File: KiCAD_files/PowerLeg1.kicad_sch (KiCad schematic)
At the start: 63 parts, among them Q301 IPD200N15N3, Q302 IPD200N15N3, Q303 IPD200N15N3, U301 AMC1100DUB, U302 ACS730xLCTR-20AB, U303 UCC21222DR, U304 OPA316, U305 OPA316, U306 SFH617A-2X009T

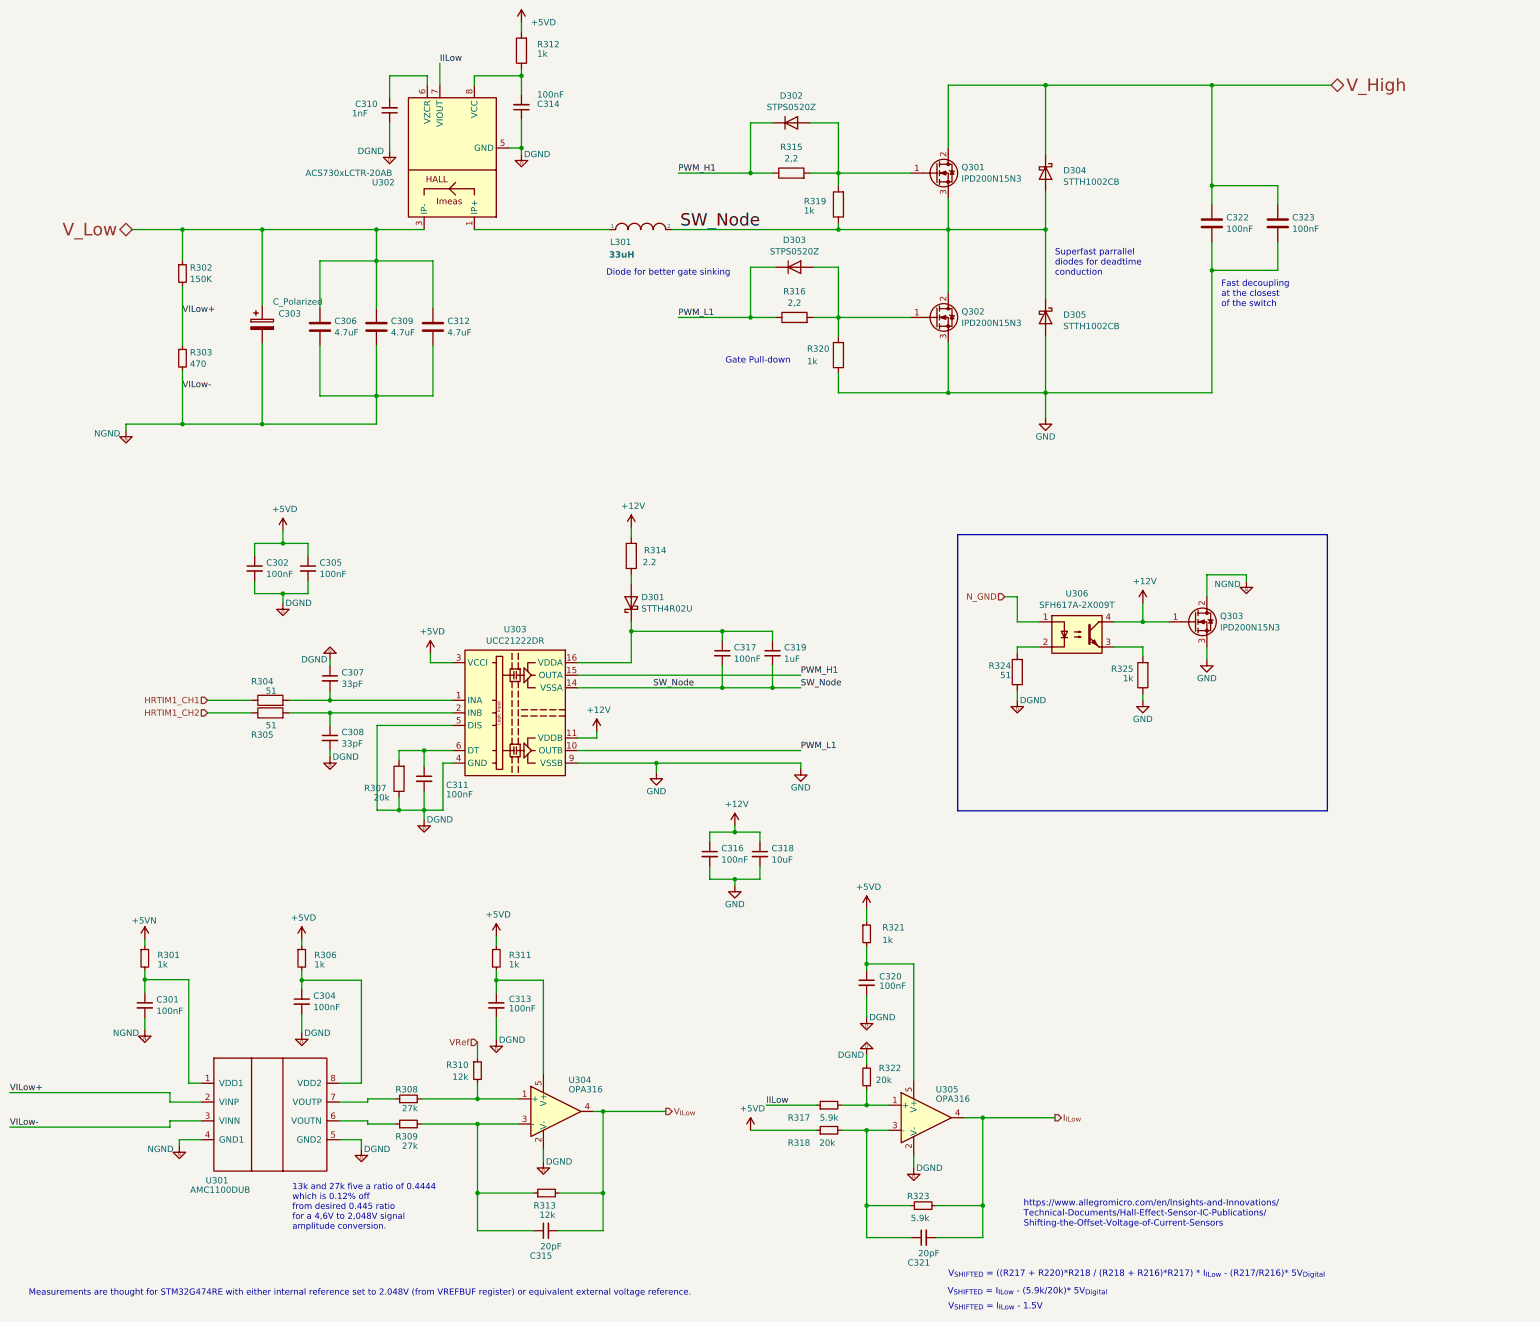
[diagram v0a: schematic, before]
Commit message: WIP: integrated the feeder on the power board directly
Former-commit-id: e81265b44c994f7ae6e14a178f616f328de7a2ab
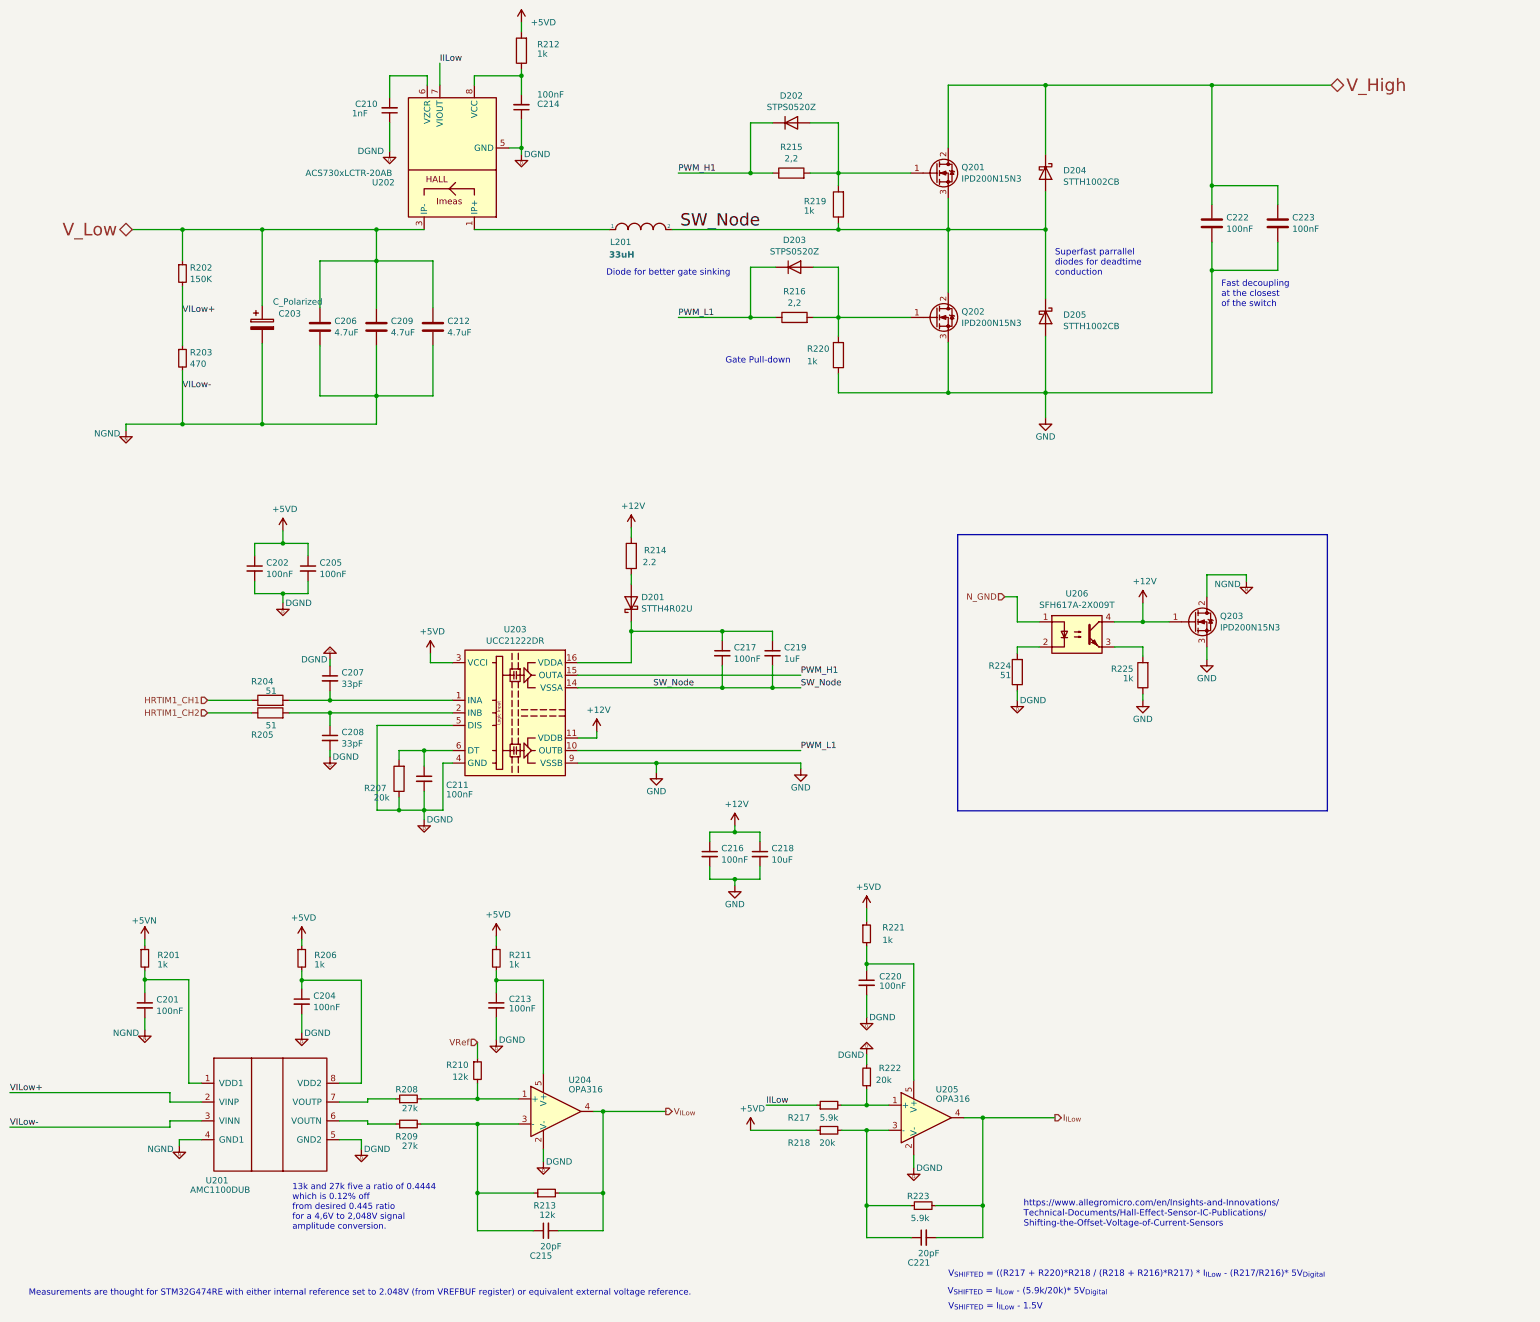
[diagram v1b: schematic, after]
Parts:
- renumbered C301 to C201, C302 to C202, C303 to C203, C304 to C204, C305 to C205, C306 to C206, C307 to C207, C308 to C208, C309 to C209, C310 to C210, C311 to C211, C312 to C212, C313 to C213, C314 to C214, C315 to C215, C316 to C216, C317 to C217, C318 to C218, C319 to C219, C320 to C220, C321 to C221, C322 to C222, C323 to C223, D301 to D201, D302 to D202, D303 to D203, D304 to D204, D305 to D205, L301 to L201, Q301 to Q201, Q302 to Q202, Q303 to Q203, R301 to R201, R302 to R202, R303 to R203, R304 to R204, R305 to R205, R306 to R206, R307 to R207, R308 to R208, R309 to R209, R310 to R210, R311 to R211, R312 to R212, R313 to R213, R314 to R214, R315 to R215, R316 to R216, R317 to R217, R318 to R218, R319 to R219, R320 to R220, R321 to R221, R322 to R222, R323 to R223, R324 to R224, R325 to R225, U301 to U201, U302 to U202, U303 to U203, U304 to U204, U305 to U205, U306 to U206

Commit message: WIP : 99 percents of the nets are now routed properly
Former-commit-id: fcbb95e3f0a6512a63faba729c3990d7109d7768
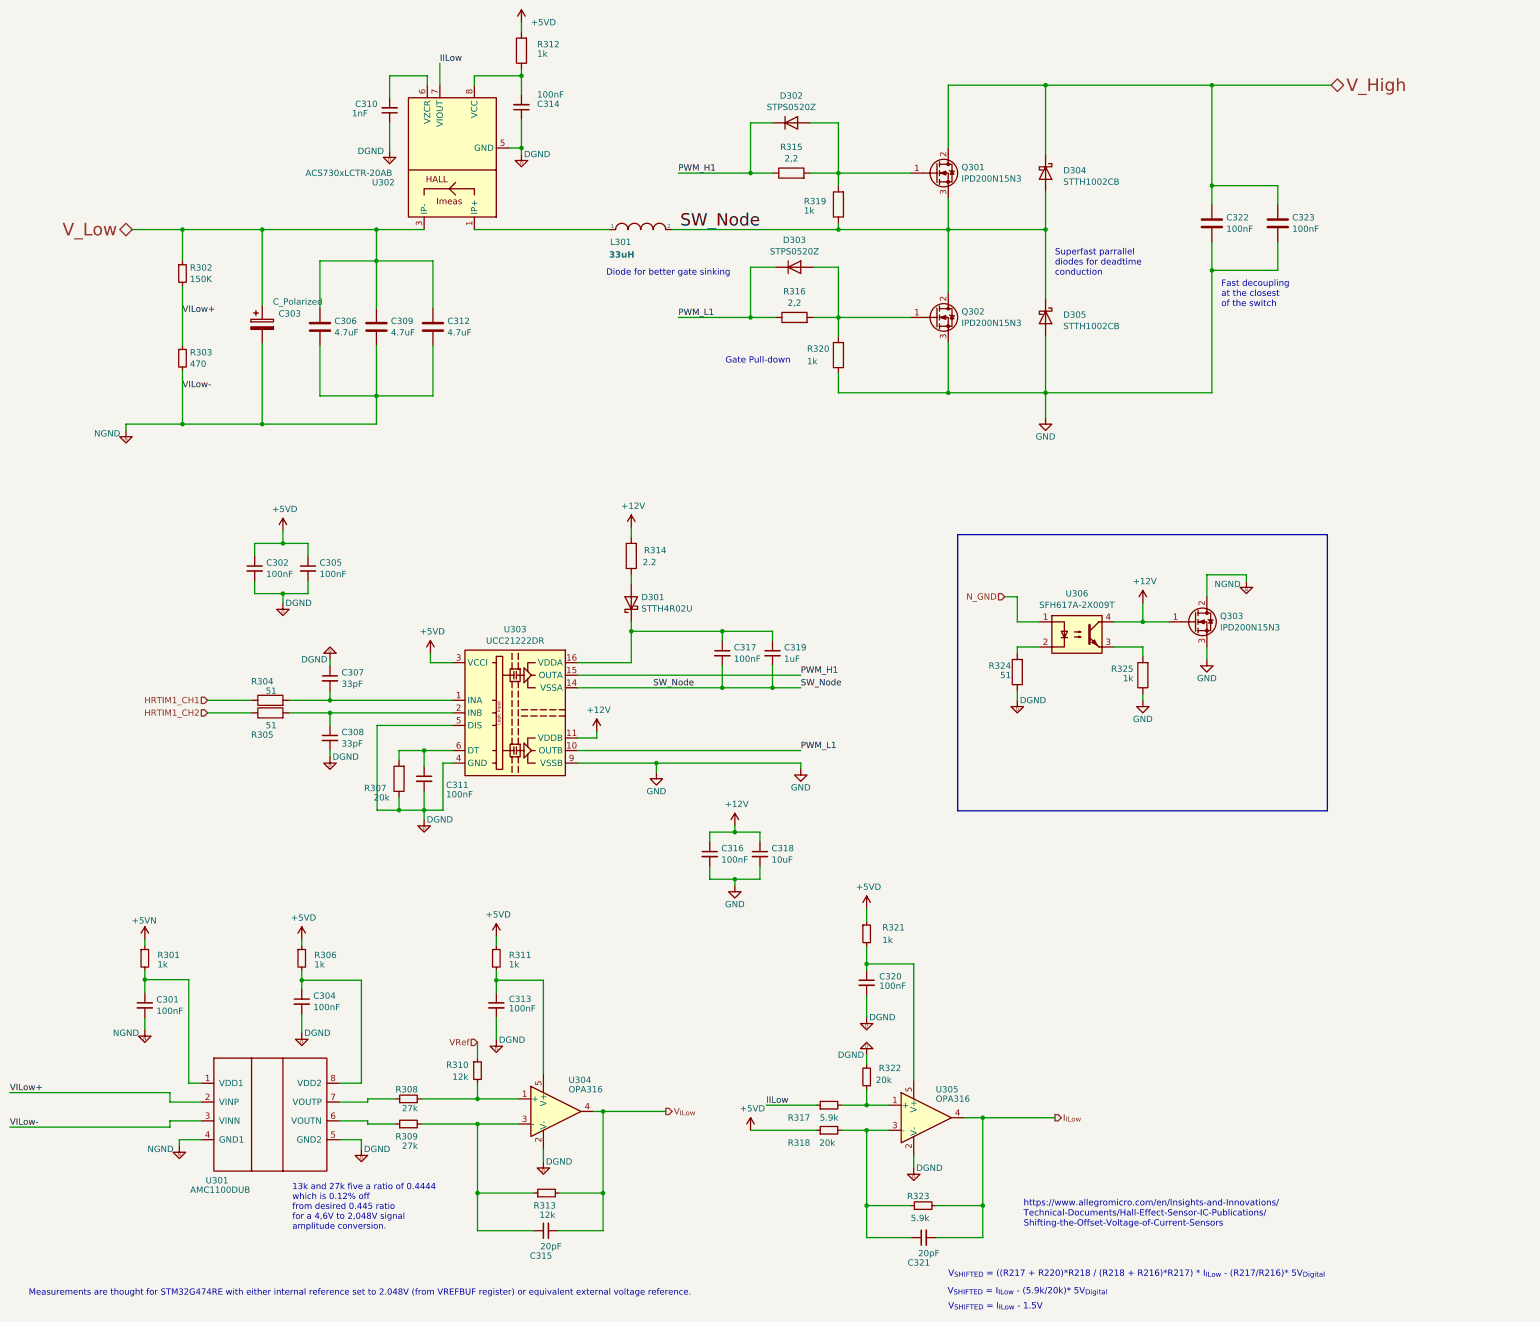
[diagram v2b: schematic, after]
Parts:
- renumbered C201 to C301, C202 to C302, C203 to C303, C204 to C304, C205 to C305, C206 to C306, C207 to C307, C208 to C308, C209 to C309, C210 to C310, C211 to C311, C212 to C312, C213 to C313, C214 to C314, C215 to C315, C216 to C316, C217 to C317, C218 to C318, C219 to C319, C220 to C320, C221 to C321, C222 to C322, C223 to C323, D201 to D301, D202 to D302, D203 to D303, D204 to D304, D205 to D305, L201 to L301, Q201 to Q301, Q202 to Q302, Q203 to Q303, R201 to R301, R202 to R302, R203 to R303, R204 to R304, R205 to R305, R206 to R306, R207 to R307, R208 to R308, R209 to R309, R210 to R310, R211 to R311, R212 to R312, R213 to R313, R214 to R314, R215 to R315, R216 to R316, R217 to R317, R218 to R318, R219 to R319, R220 to R320, R221 to R321, R222 to R322, R223 to R323, R224 to R324, R225 to R325, U201 to U301, U202 to U302, U203 to U303, U204 to U304, U205 to U305, U206 to U306
